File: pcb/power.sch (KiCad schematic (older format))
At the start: 41 parts, among them P8 CONN_01X06, P9 CONN_01X02, U1 TPS2420, U2 LT3487, U3 TPS63002, U7 TPS56x200, U8 LMZ10500

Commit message: Safety checkin.
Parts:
- removed C11: 10uF, Capacitors_SMD:C_0805_HandSoldering, symbol C
- removed C25: 47uF, Capacitors_SMD:C_1206_HandSoldering, symbol C
- removed C4: 2.2uF, Capacitors_SMD:C_0603_HandSoldering, symbol C
- removed L3: 2.0uH, w_smd_inductors:inductor_smd_0805, symbol INDUCTOR
- removed P8: CONN_01X06, Pin_Headers:Pin_Header_Straight_1x06, symbol CONN_01X06
- removed P9: CONN_01X02, Pin_Headers:Pin_Header_Straight_1x02, symbol CONN_01X02
- removed U3: TPS63002, Housings_DFN_QFN:DFN-10-1EP_3x3mm_Pitch0.5mm, symbol TPS63002
- added C11: 0.1uF, Capacitors_SMD:C_0805_HandSoldering, symbol Device:C_Small
- added C13, C17, C18, C19, C50: 10.0uF, Capacitors_SMD:C_0805_HandSoldering, symbol Device:C
- added C22, C23, C25, C4, C52: 10uF, Capacitors_SMD:C_0805_HandSoldering, symbol Device:C
- added C24: 0.47uF, Capacitors_SMD:C_0805_HandSoldering, symbol Device:C_Small
- added C51: 4.7uF, Capacitors_SMD:C_0805_HandSoldering, symbol Device:C
- added NT1: Net-Tie_3, symbol Device:Net-Tie_3
- added R10: 200K, Resistors_SMD:R_0402, symbol Device:R_Small
- added R11: 49K9, Resistors_SMD:R_0402, symbol Device:R_Small
- added R12: 499R, Resistors_SMD:R_0402, symbol Device:R_Small
- added R13: 487K, Resistors_SMD:R_0402, symbol Device:R_Small
- added R14: 100K, Resistors_SMD:R_0402, symbol Device:R_Small
- added U12: LT3042, Package_DFN_QFN:DFN-10-1EP_3x3mm_P0.5mm_EP1.65x2.38mm_ThermalVias, symbol @Engstad:LT3042
- added U3: TPS7A3401, symbol @Engstad:TPS7A3401
- added U9: RT9069-C0GB, Package_TO_SOT_SMD:SOT-23-5, symbol @Engstad:RT9069-C0GB
- C1, C10, C15, C2, C21, C3, C6, C7, C9: symbol C -> Device:C
- C14: value 10.0uF -> 10uF; symbol C_Small -> Device:C
- C16, C20: symbol C_Small -> Device:C_Small
- C5: symbol C -> Device:C_Small
- C8: value 1.0uF/11mOhm -> 1.0uF; symbol C -> Device:C
- D1: symbol ZENER -> Device:D_Zener_ALT
- L1, L8: symbol L_Small -> Device:L
- L2, L4: symbol L_Small -> Device:L_Small
- R1, R3, R4, R5, R6: symbol R -> Device:R
- R16, R17, R8, R9: symbol R_Small -> Device:R_Small
- R2: value 324k -> 324K; symbol R -> Device:R_Small
- R7: value 324k -> 487K; symbol R -> Device:R_Small
- U1: footprint Housings_DFN_QFN:QFN-16-1EP_4x4mm_Pitch0.65mm -> Package_DFN_QFN:QFN-16-1EP_4x4mm_P0.65mm_EP2.7x2.7mm_ThermalVias; symbol TPS2420 -> @Engstad:TPS2420
- U2: footprint w_smd_qfn:dfn10-3x3 -> Package_DFN_QFN:DFN-10-1EP_3x3mm_P0.5mm_EP1.7x2.5mm; symbol LT3487 -> @Engstad:LT3487
- U7: footprint Housings_SOT-23_SOT-143_TSOT-6:SOT-23-6 -> Package_TO_SOT_SMD:SOT-23-6; symbol TPS56x200 -> @Engstad:TPS56x200
- U8: footprint camera:llp-8 -> Engstad:Texas_Instruments-LLP-8; symbol LMZ10500 -> @Engstad:LMZ10500
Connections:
- net labels added: +12VA, +1V8, +3V3, +5VA, -8V, 13V5, GNDA, GNDPWR, IGND
- net labels removed: +12V, 12V, 1V8, 3V3, 5V0
- wire segments 137 -> 227
- no-connect marks 1 -> 2
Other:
- note added: "250 mA max"
- note added: "I_lim = 125 mA * 1 kOhm / R_ilim\nR_ilim = 125 mA * 1 kOhm / I_ilim"
- note added: "Iout = 100mA\nMax power dissipation = 0.45W\n100 mA * 1.5 V = 0.15W\n"
- note added: "Iout = 2A"
- note added: "Power grounds should be connected close to the supply.\nAnalog grounds should be connected close to the load."
- note added: "R1 = (13.2V - 1.23V) / 25 uA = 490.8 K = 487K\n25e-6 * 497e3 + 1.23 = 13.65 V."
- note added: "R2 = - Vneg / 25 uA = 8V / 25 uA = 320K\n-324K * 25 uA = -8.1 V"
- note added: "TODO: Need 1.8VA"
- note added: "Vin: 3V to 12V"
- note added: "|Vfb| / R2 > 5 uA => R2 < 1.184 V / 5 uA = 237K\nR1 = R2 * (Vo / Vfb - 1) = 100K * ((-7.0) / (-1.184) - 1.0) = 491.2K = 487K\n"
- moved on the sheet: U1, U2, U7

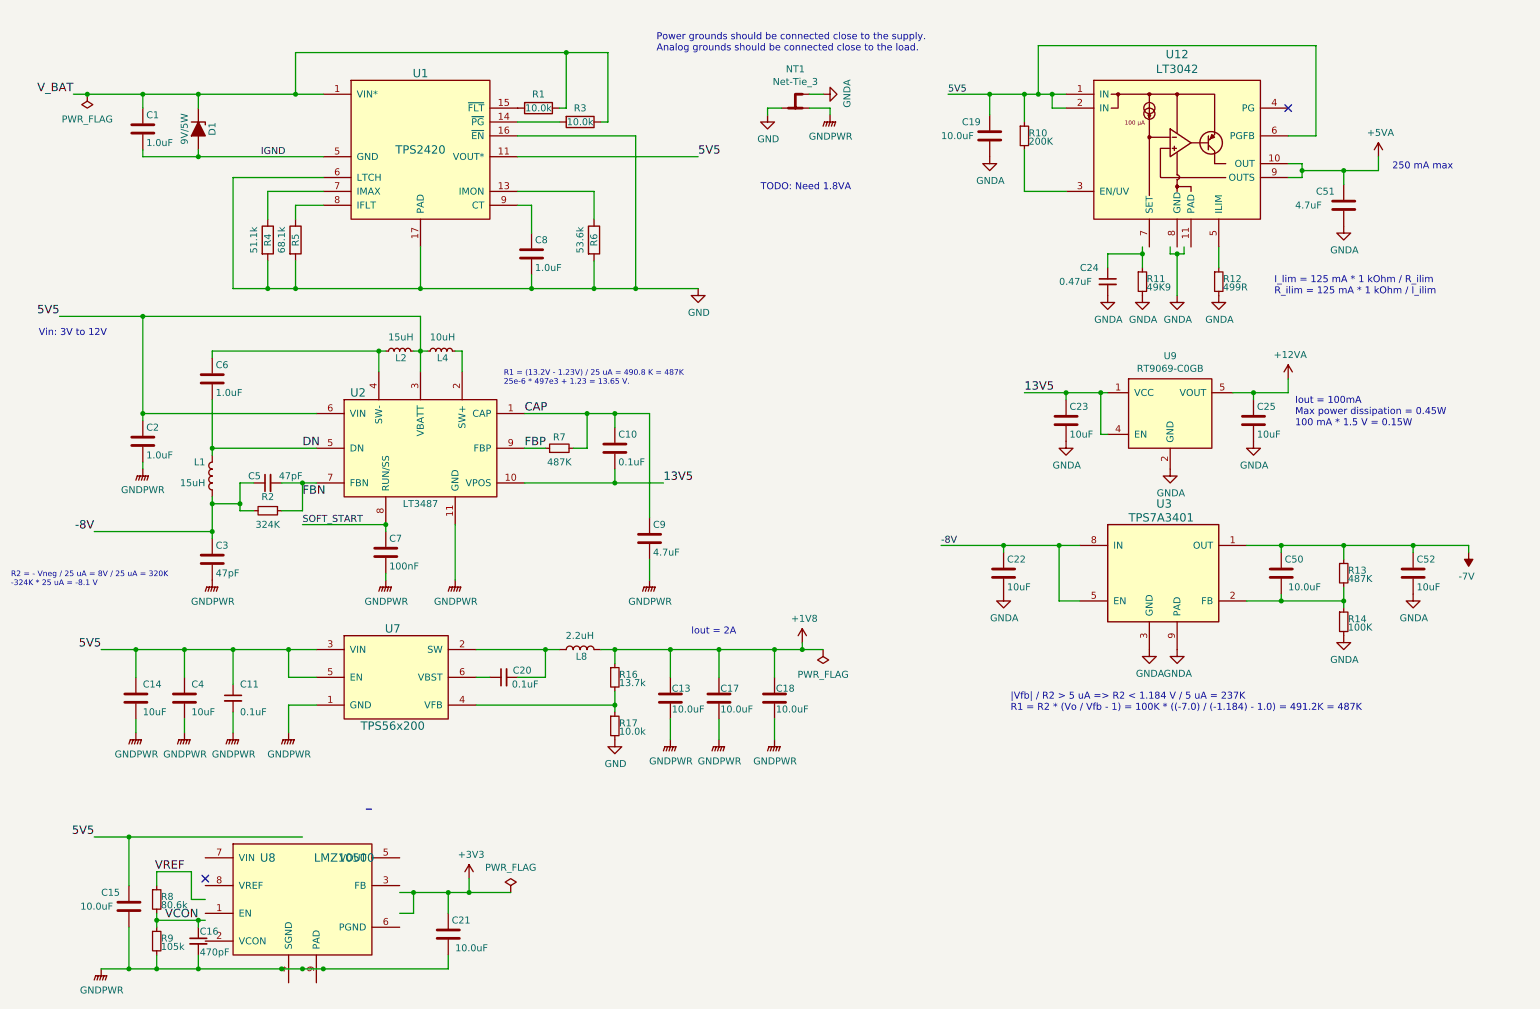
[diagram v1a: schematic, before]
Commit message: A little more work.
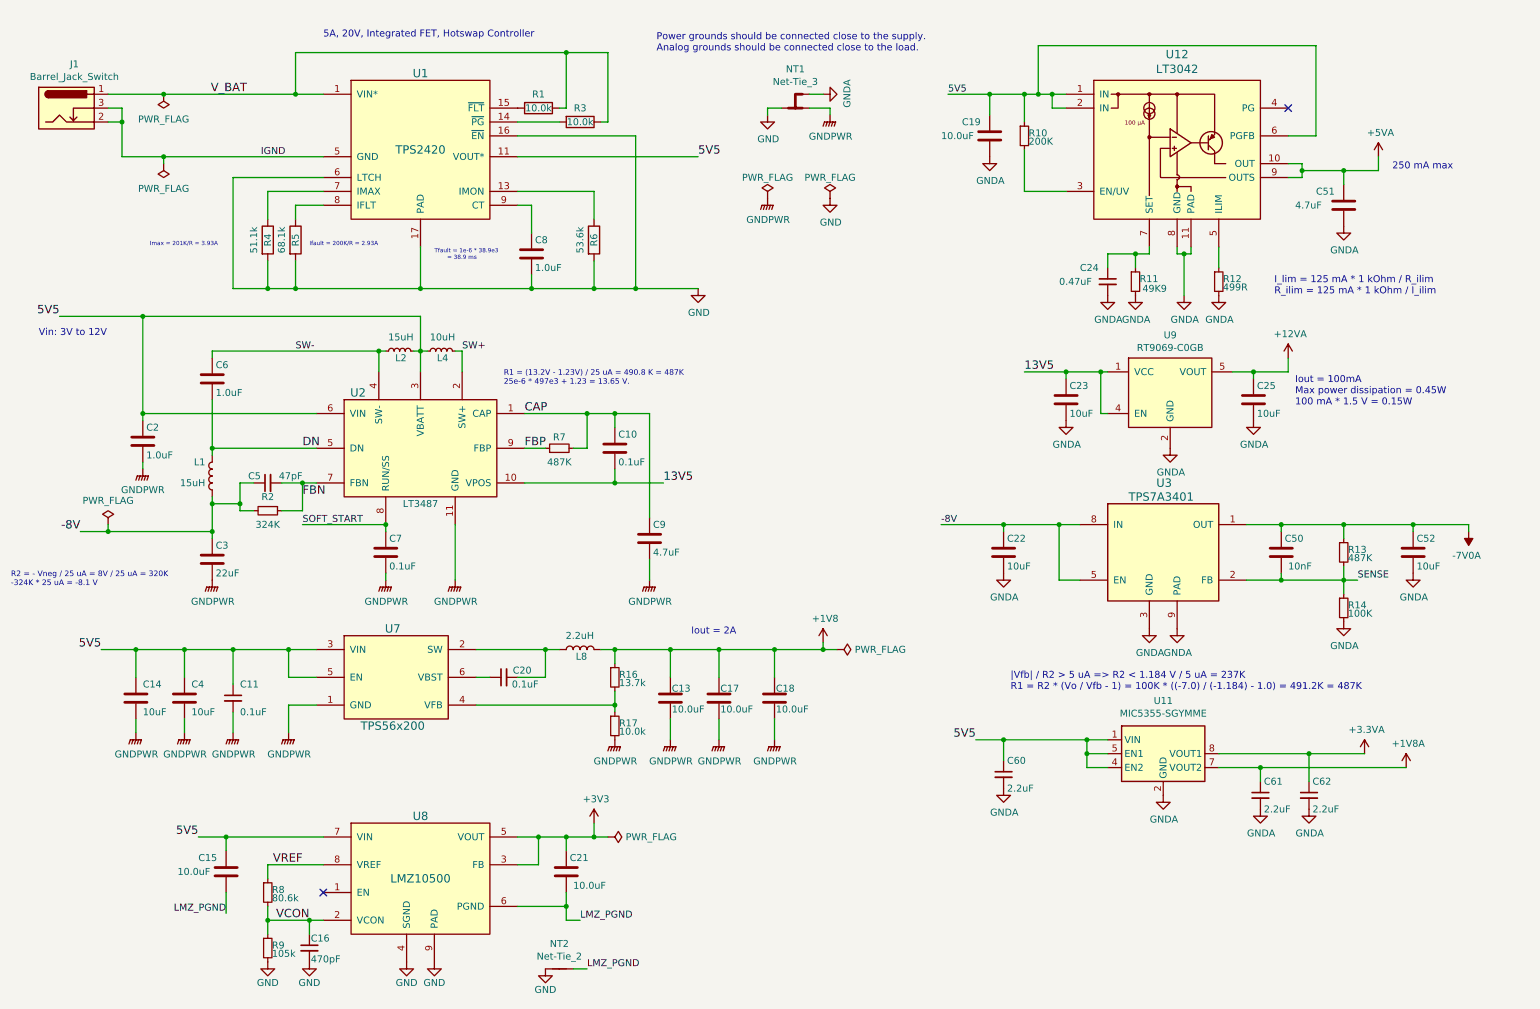
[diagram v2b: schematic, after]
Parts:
- removed C1: 1.0uF, Capacitors_SMD:C_0805_HandSoldering, symbol Device:C
- removed D1: 9V/5W, Diodes_SMD:Diode-SMB_Handsoldering, symbol Device:D_Zener_ALT
- added C60, C61, C62: 2.2uF, Capacitor_SMD:C_0603_1608Metric, symbol Device:C_Small
- added J1: Barrel_Jack_Switch, symbol Connector:Barrel_Jack_Switch
- added NT2: Net-Tie_2, NetTie:NetTie-2_THT_Pad0.3mm, symbol Device:Net-Tie_2
- added U11: MIC5355-SGYMME, Package_SO:MSOP-8-1EP_3x3mm_P0.65mm_EP2.5x3mm_Mask1.73x2.36mm_ThermalVias, symbol Regulator_Linear:MIC5355-SGYMME
- C10, C11, C2, C24, C5, C6, C8: footprint Capacitors_SMD:C_0805_HandSoldering -> Capacitor_SMD:C_0603_1608Metric
- C13, C17, C18, C19, C22, C23, C25, C52: footprint Capacitors_SMD:C_0805_HandSoldering -> Capacitor_SMD:C_1206_3216Metric
- C14, C15, C21, C4, C51, C9: footprint Capacitors_SMD:C_0805_HandSoldering -> Capacitor_SMD:C_0805_2012Metric
- C16: footprint Capacitors_SMD:C_0402 -> Capacitor_SMD:C_0603_1608Metric
- C20: footprint Capacitors_SMD:C_0603_HandSoldering -> Capacitor_SMD:C_0603_1608Metric
- C3: value 47pF -> 22uF; footprint Capacitors_SMD:C_0805_HandSoldering -> Capacitor_SMD:C_1206_3216Metric
- C50: value 10.0uF -> 10nF; footprint Capacitors_SMD:C_0805_HandSoldering -> Capacitor_SMD:C_0603_1608Metric
- C7: value 100nF -> 0.1uF; footprint Capacitors_SMD:C_0805_HandSoldering -> Capacitor_SMD:C_0603_1608Metric
- L1, L2, L4: footprint w_smd_inductors:inductor_smd_0805 -> Engstad:L_Wurth-4018
- L8: footprint w_smd_inductors:inductor_smd_0805 -> Inductor_SMD:L_0805_2012Metric
- NT1: footprint (none) -> NetTie:NetTie-3_SMD_Pad0.5mm
- R1: footprint Resistors_SMD:R_0805_HandSoldering -> Resistor_SMD:R_0603_1608Metric
- R10, R11, R12, R13, R14, R16, R17, R8, R9: footprint Resistors_SMD:R_0402 -> Resistor_SMD:R_0603_1608Metric
- R2, R3, R4, R5, R6, R7: footprint Resistors_SMD:R_0603_HandSoldering -> Resistor_SMD:R_0603_1608Metric
- U3: footprint (none) -> Engstad:VSSOP-8_3.0x3.0mm_P0.65mm
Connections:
- net labels added: +1V8A, +3.3VA, -7V0A, LMZ_PGND, SENSE, SW+, SW-
- net labels removed: -7V
- wire segments 227 -> 237
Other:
- note added: "5A, 20V, Integrated FET, Hotswap Controller"
- note added: "Ifault = 200K/R = 2.93A"
- note added: "Imax = 201K/R = 3.93A"
- note added: "Tfault = 1e-6 * 38.9e3 \n = 38.9 ms"
- note removed: "TODO: Need 1.8VA"
- moved on the sheet: C15, C16, C21, C22, C23, C25, C50, C52, R11, R13, R14, R8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
